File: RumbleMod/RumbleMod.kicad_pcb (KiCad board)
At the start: 2 copper layers, 38.1 x 48.9 mm, 10 parts, among them J1 Screw_Terminal_01x02, J2 Screw_Terminal_01x01, J3 Screw_Terminal_01x02, J4 Screw_Terminal_01x02, Q1 2N3904, U1 LM741, U2 LM555xN

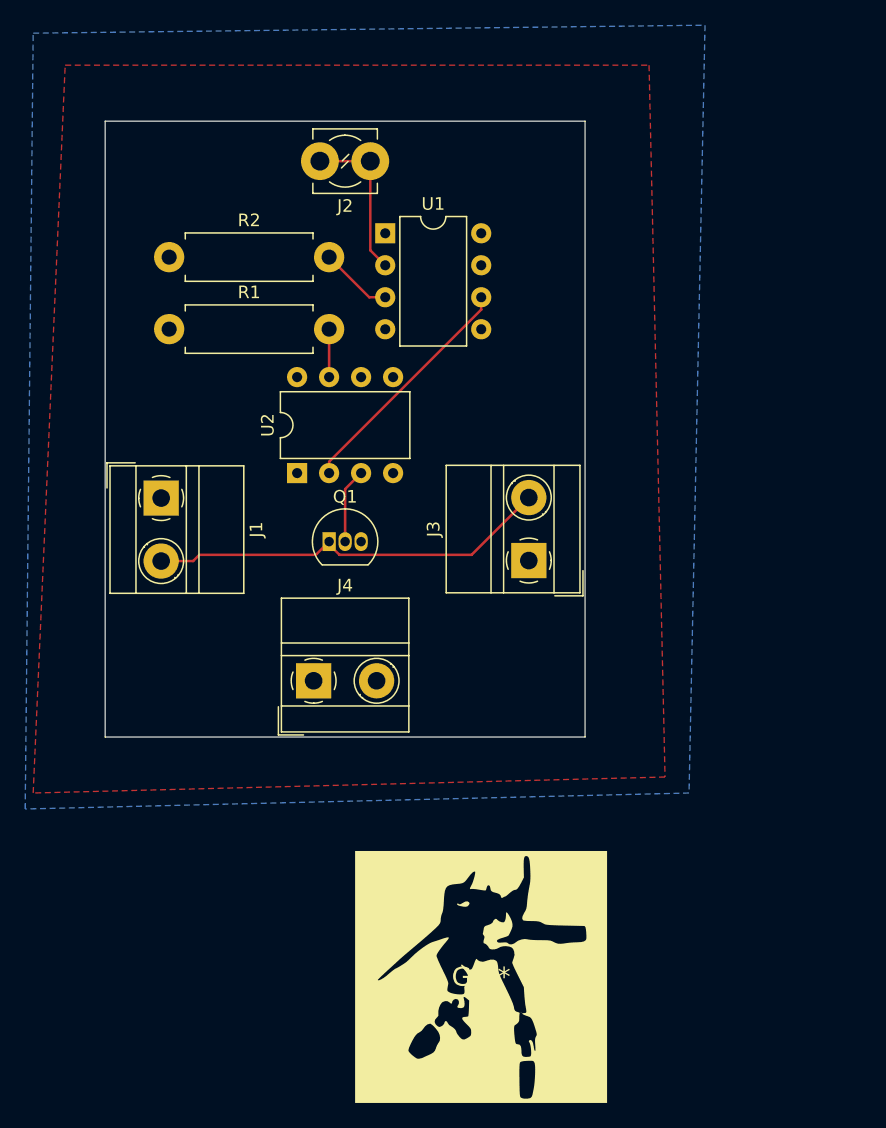
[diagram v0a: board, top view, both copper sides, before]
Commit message: Add production
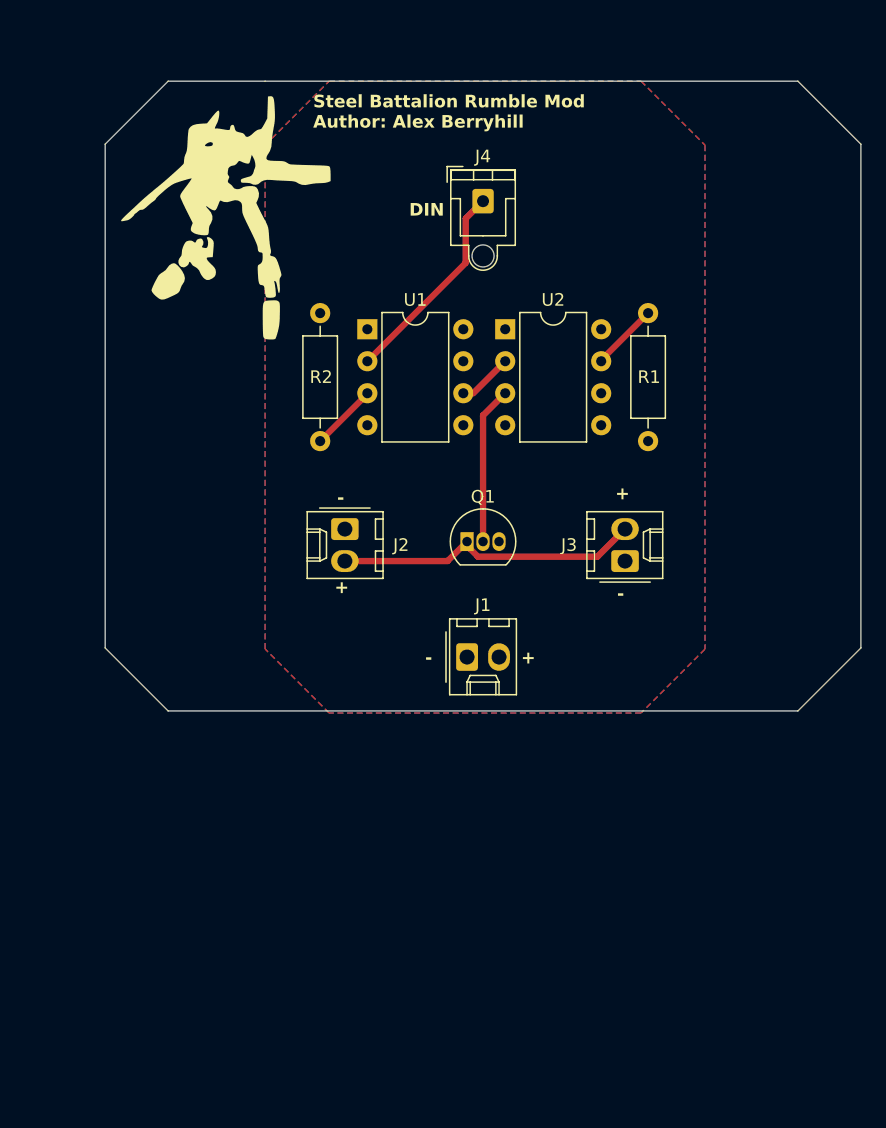
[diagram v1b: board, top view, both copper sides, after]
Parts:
- J1, J3: value Screw_Terminal_01x02 -> Conn_01x02; footprint TerminalBlock_MetzConnect:TerminalBlock_MetzConnect_Type011_RT05502HBWC_1x02_P5.00mm_Horizontal -> Connector_Molex:Molex_KK-254_AE-6410-02A_1x02_P2.54mm_Vertical
- J2: value Screw_Terminal_01x01 -> Conn_01x02; footprint TerminalBlock_MetzConnect:TerminalBlock_MetzConnect_360381_1x01_Horizontal_ScrewM3.0 -> Connector_Molex:Molex_KK-254_AE-6410-02A_1x02_P2.54mm_Vertical
- J4: value Screw_Terminal_01x02 -> Conn_01x01_Socket; footprint TerminalBlock_MetzConnect:TerminalBlock_MetzConnect_Type011_RT05502HBWC_1x02_P5.00mm_Horizontal -> Connector_JST:JST_XH_B1B-XH-AM_1x01_P2.50mm_Vertical
- R1, R2: footprint Resistor_THT:R_Axial_DIN0411_L9.9mm_D3.6mm_P12.70mm_Horizontal -> Resistor_THT:R_Axial_DIN0207_L6.3mm_D2.5mm_P10.16mm_Horizontal
- moved G*** 63.7 mm to (156.2, 68.6)
- moved J4 40.4 mm to (176.7, 67.3)
- moved R1 39.1 mm to (189.8, 86.4), turned to 90 degrees
- moved J2 29.3 mm to (165.7, 93.3), turned to -90 degrees
- moved J1 27.4 mm to (175.4, 103.5), turned to 0 degrees
- moved U2 20.1 mm to (178.4, 77.5), turned to 0 degrees
- moved R2 12.8 mm to (163.8, 76.2), turned to -90 degrees
- moved Q1 10.9 mm to (175.4, 94.3)
- moved U1 7.75 mm to (167.5, 77.5)
- moved J3 7.64 mm to (188.0, 95.9)
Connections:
- J1 pad 2: Net-(J1-Pin_2) -> +5V
- J2 pad 1: Net-(J2-Pin_1) -> GND
- J3 pad 2: Net-(J1-Pin_2) -> Net-(J2-Pin_2)
- J4 pad 1: GND -> Net-(J4-Pin_1)
- Q1 pad 1: Net-(J1-Pin_2) -> Net-(J2-Pin_2)
- U1 pad 2: Net-(J2-Pin_1) -> Net-(J4-Pin_1)
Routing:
- net Net-(J1-Pin_2): track 32.3 -> 0.00 mm
- net Net-(J2-Pin_2): track 0.00 -> 24.5 mm
- net Net-(J4-Pin_1): track 0.00 -> 16.5 mm
- net Net-(U2-TR): track 19.0 -> 4.38 mm
- net Net-(J2-Pin_1): track 12.8 -> 0.00 mm
- net Net-(Q1-B): track 6.43 -> 13.0 mm
- net Net-(U2-DIS): track 3.81 -> 5.36 mm
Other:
- board size 38.1 x 48.9 mm -> 60 x 50 mm
- board text added: "+"
- board text added: "-"
- board text added: "DIN"
- board text added: "Steel Battalion Rumble Mod Author: Alex Berryhill"

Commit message: new production files
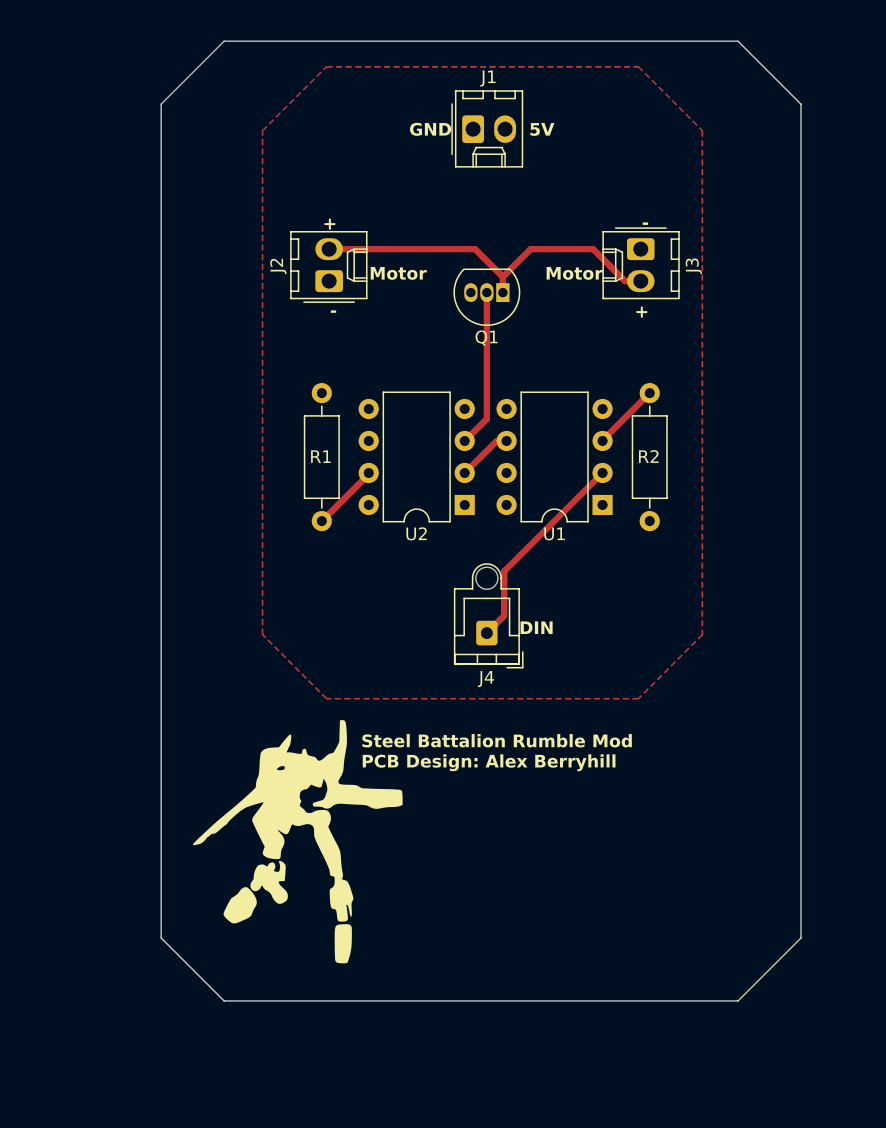
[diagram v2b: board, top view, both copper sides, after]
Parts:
- moved G*** 49.9 mm to (161.9, 118.1)
- moved J1 41.9 mm to (175.9, 61.6)
- moved J4 34.3 mm to (177.0, 101.6), turned to 180 degrees
- moved R2 30.9 mm to (189.9, 92.7), turned to 90 degrees
- moved R1 26.2 mm to (163.9, 82.5), turned to -90 degrees
- moved J3 24.8 mm to (189.2, 71.1), turned to -90 degrees
- moved U1 23.3 mm to (186.2, 91.4), turned to 180 degrees
- moved Q1 20.0 mm to (178.3, 74.6), turned to 180 degrees
- moved J2 19.7 mm to (164.5, 73.7), turned to 90 degrees
- moved U2 14.3 mm to (175.2, 91.4), turned to 180 degrees
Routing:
- net Net-(J2-Pin_2): track 24.5 -> 28.3 mm
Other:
- board size 60 x 50 mm -> 50.8 x 76.2 mm
- board text added: "5V"
- board text added: "GND"
- board text added: "Motor"
- board text added: "Steel Battalion Rumble Mod PCB Design: Alex Berryhill"
- board text removed: "Steel Battalion Rumble Mod Author: Alex Berryhill"
